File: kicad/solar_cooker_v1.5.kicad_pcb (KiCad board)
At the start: 2 copper layers, 160.5 x 77.2 mm, 20 parts, among them J1 Pt100, J2 microSD, J3 clock_module, J4 Pt100, J5 BME680, J6 GPS, J7 Pt100, J8 display, U1 anemometer, U2 AM2315C, U3 pyranometer

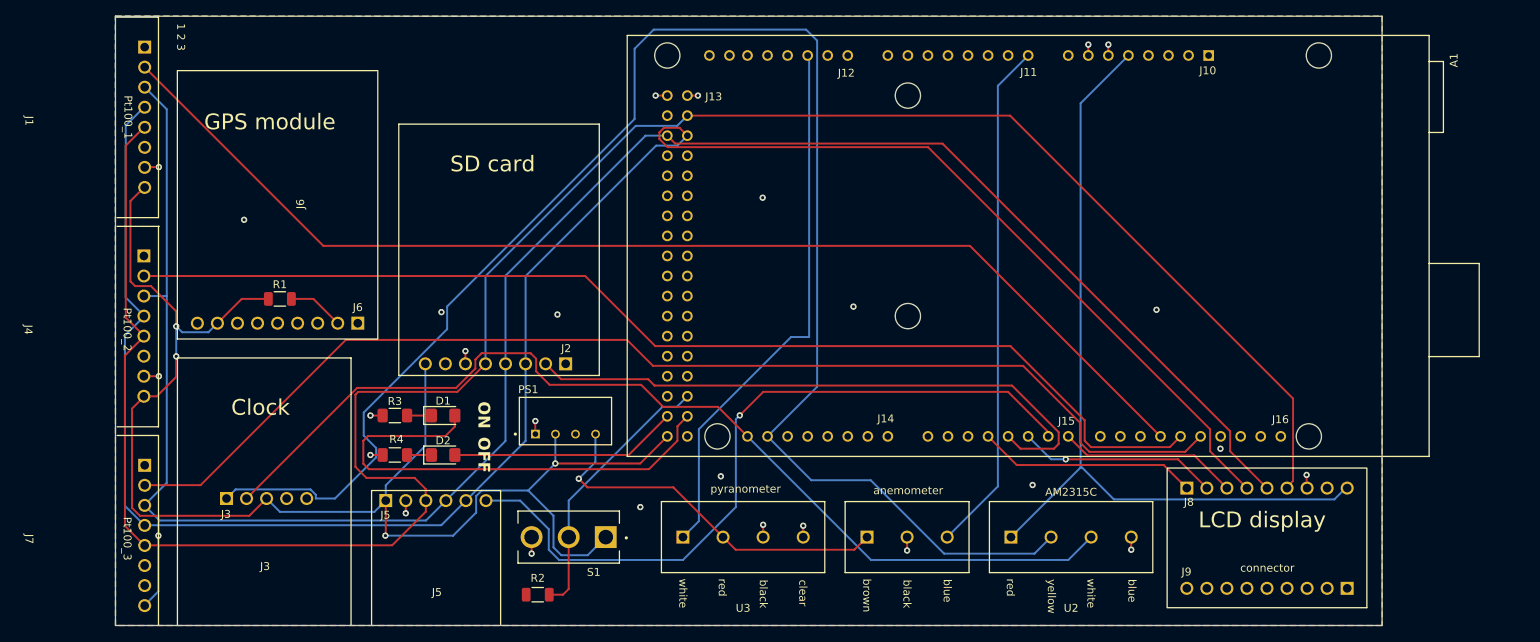
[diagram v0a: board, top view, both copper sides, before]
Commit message: footprints update
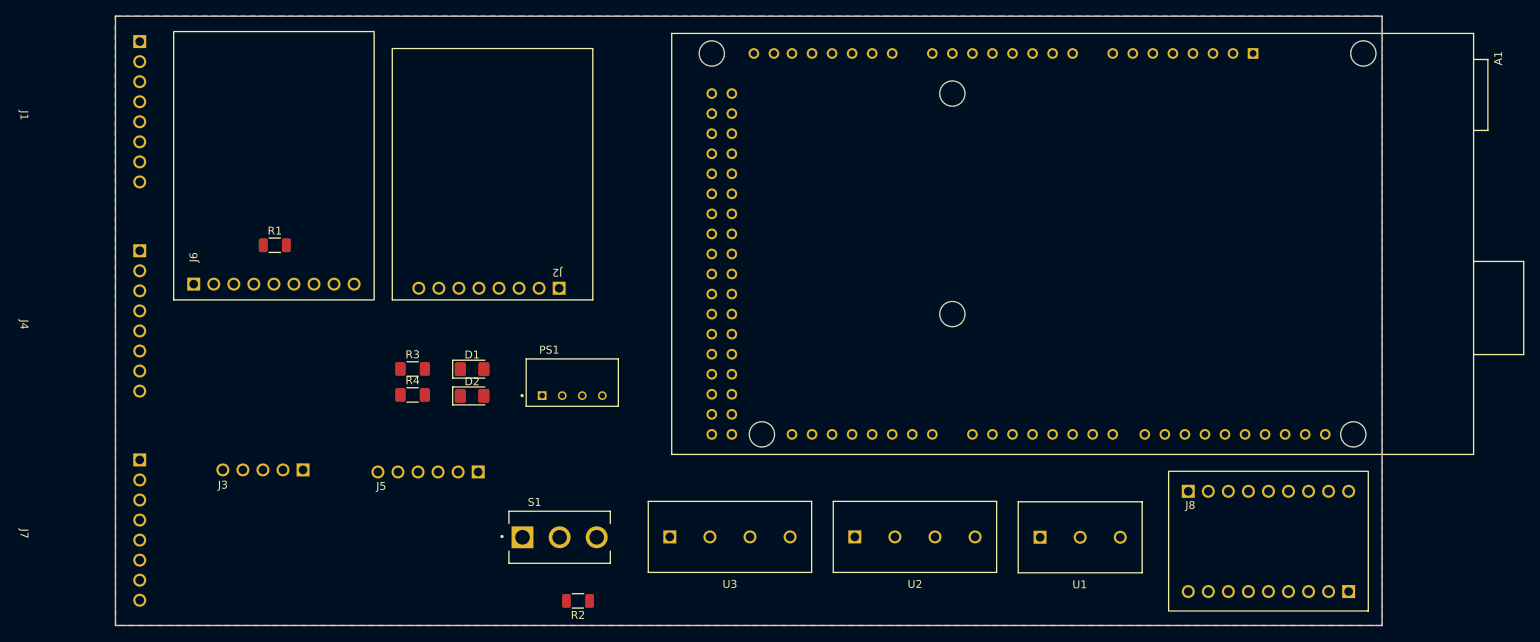
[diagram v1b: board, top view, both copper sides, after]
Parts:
- moved U1 21.9 mm to (192.3, 146.0)
- moved U2 19.8 mm to (171.4, 146.0)
- moved J2 9.61 mm to (117.9, 98.2)
- moved D2 8.34 mm to (115.3, 128.1)
- moved R4 7.93 mm to (107.8, 128.0), turned to 0 degrees
- moved D1 6.93 mm to (115.3, 124.7)
- moved R1 6.83 mm to (90.3, 109.0), turned to 0 degrees
- moved R3 6.31 mm to (107.8, 124.7), turned to 0 degrees
- moved A1 5.64 mm to (191.4, 108.9)
- moved R2 5.16 mm to (128.7, 154.1), turned to 180 degrees
- moved J6 4.97 mm to (90.2, 99.0)
- moved PS1 4.95 mm to (128.0, 126.4)
- moved J5 3.77 mm to (109.7, 145.8)
- moved J3 3.65 mm to (88.8, 137.4)
- moved U3 1.67 mm to (148.0, 146.0)
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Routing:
- net +5V: track 298.2 -> 0.00 mm, vias 5 -> 0
- net /SCK: track 282.9 -> 0.00 mm
- net /MISO: track 257.8 -> 0.00 mm
- net /MOSI: track 253.5 -> 0.00 mm
- net /SDA: track 209.4 -> 0.00 mm
- net /D13: track 149.6 -> 0.00 mm
- net /D11: track 148.1 -> 0.00 mm
- net /D12: track 142.4 -> 0.00 mm
- net /SCL: track 128.3 -> 0.00 mm
- net /D6: track 93.9 -> 0.00 mm, vias 1 -> 0
- net /D4: track 77.4 -> 0.00 mm
- net /A10: track 69.1 -> 0.00 mm
- net /A0: track 65.3 -> 0.00 mm
- net /D22: track 61.9 -> 0.00 mm
- net +9V: track 47.4 -> 0.00 mm, vias 1 -> 0
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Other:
- board text removed: "1 2 3"
- board text removed: "Clock"
- board text removed: "GPS module"
- board text removed: "J10"
- board text removed: "J11"
- board text removed: "J12"
- board text removed: "J13"
- board text removed: "J14"
- board text removed: "J15"
- board text removed: "J16"
- board text removed: "J9"
- board text removed: "LCD display"
- board text removed: "OFF"
- board text removed: "ON"
- board text removed: "Pt100_1"
- board text removed: "Pt100_2"
- board text removed: "Pt100_3"
- board text removed: "SD card"
- board text removed: "black"
- board text removed: "blue"
- board text removed: "brown"
- board text removed: "clear"
- board text removed: "connector"
- board text removed: "red"
- board text removed: "white"
- board text removed: "yellow"
